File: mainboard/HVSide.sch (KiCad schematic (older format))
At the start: 66 parts, among them J11 CONN_2X2, J17 HV, J18 CONN_1X2, J19 CONN_1X2, J4 CONN_2X2, U10 DCDC_ISO_5V_ISO, U15 CD4082, U16 ADCMP350, U19 TCMT1103, U23 CD4072BPW, U24 LM358, U26 TCMT1103, U27 DCDC_ISO_5V, U28 MIC5365-3.3YC5, U29 Si8900, U30 MAX14878AWA+, U7 ADCMP354

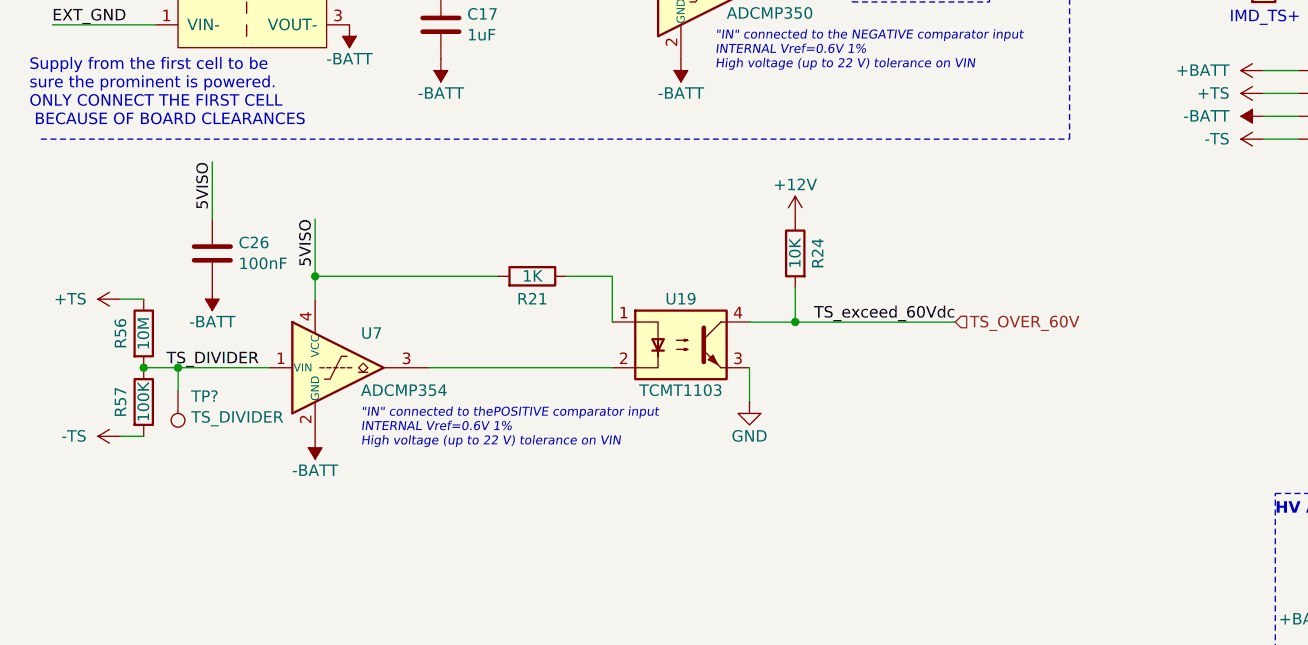
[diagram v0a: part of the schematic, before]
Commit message: minor changes
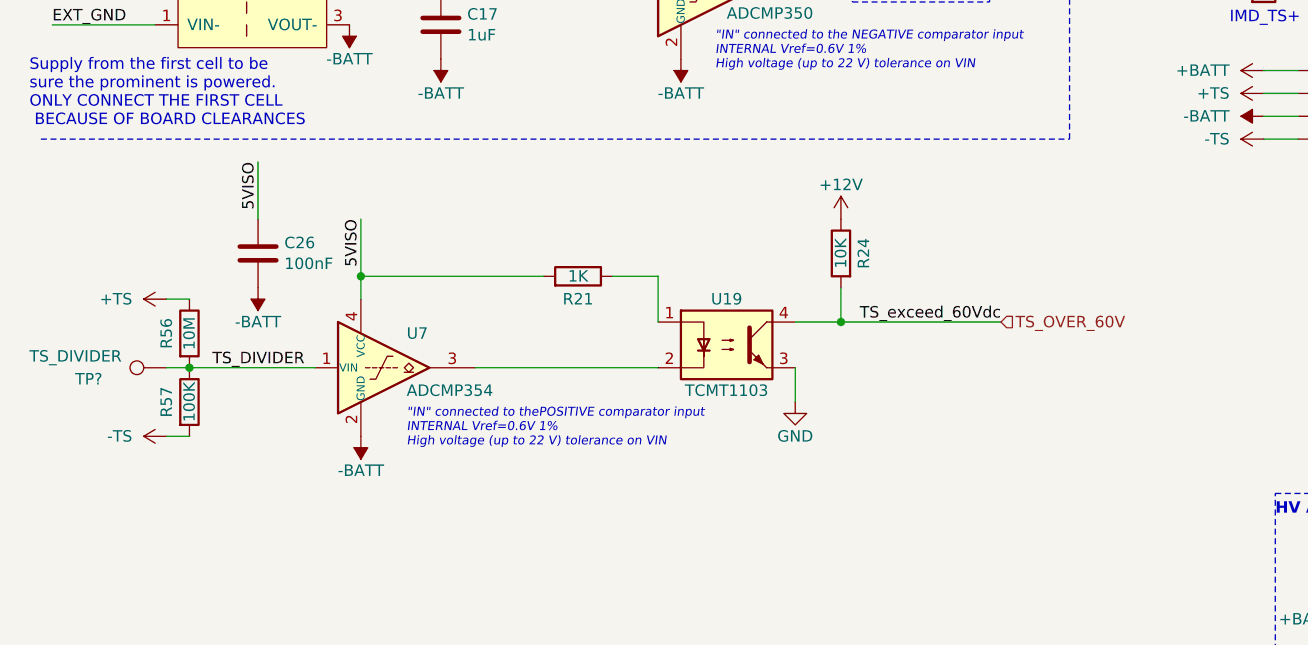
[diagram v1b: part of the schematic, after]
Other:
- moved on the sheet: C26, R21, R24, R56, R57, TP?, U19, U7
